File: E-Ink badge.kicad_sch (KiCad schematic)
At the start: 40 parts, among them J1 USB_C_Receptacle_USB2.0_14P, J2 E-INK-FPC, Q1 BSS138, SW1 BOOTSEL, SW2 RUN, SW3 W, SW4 A, SW5 S, SW6 D, U1 RP2040, U2 AP2112K-3.3, U3 W25Q16JVSS, Y1 Crystal

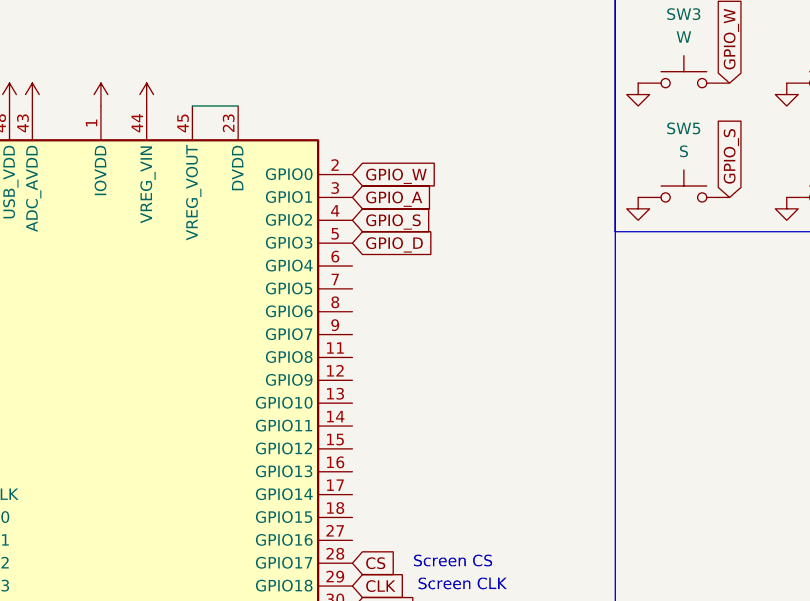
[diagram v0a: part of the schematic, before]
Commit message: Finally finished routing the whole board!
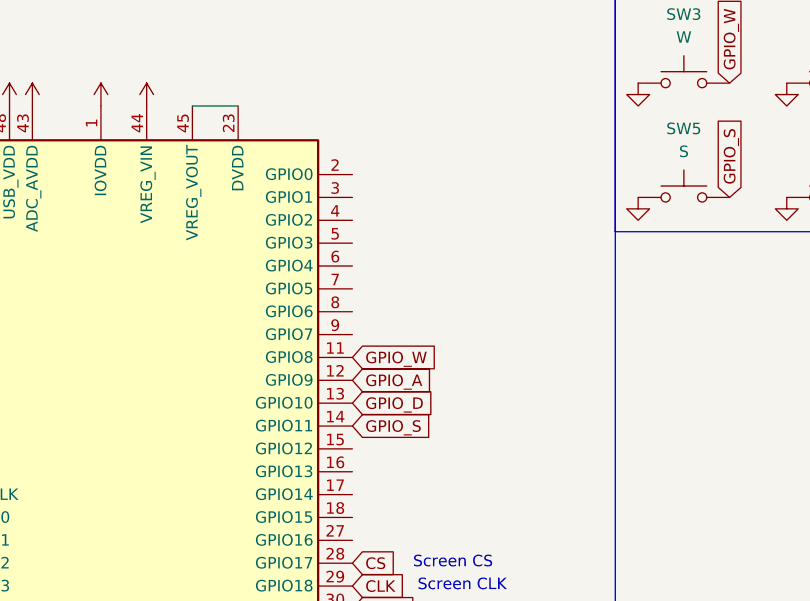
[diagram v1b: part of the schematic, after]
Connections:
- net GPIO_A: now also U1.12 (GPIO9); no longer U1.3 (GPIO1)
- net GPIO_D: now also U1.13 (GPIO10); no longer U1.5 (GPIO3)
- net GPIO_S: now also U1.14 (GPIO11); no longer U1.4 (GPIO2)
- net GPIO_W: now also U1.11 (GPIO8); no longer U1.2 (GPIO0)
